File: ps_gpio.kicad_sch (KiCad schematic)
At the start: 12 parts, among them U1 XC7Z010-1CLG400C

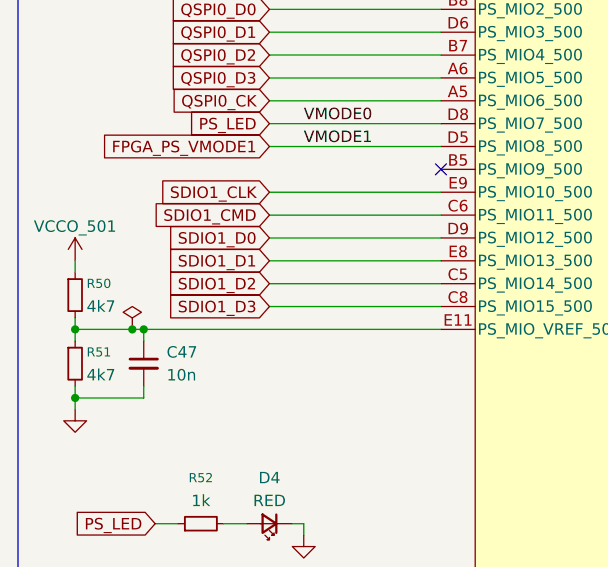
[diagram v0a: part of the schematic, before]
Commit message: update
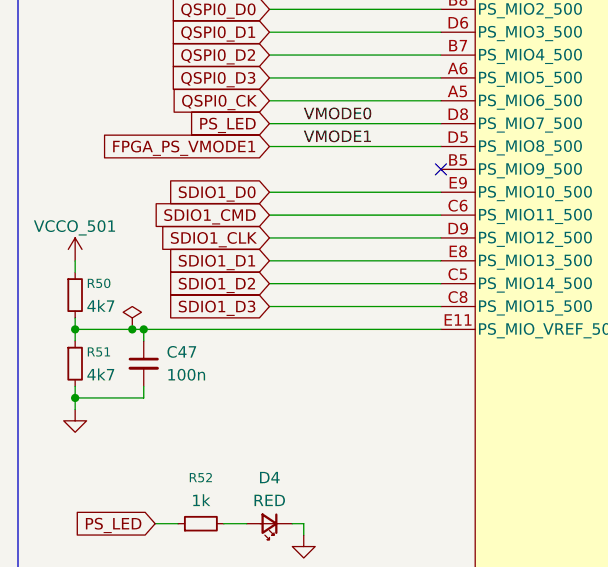
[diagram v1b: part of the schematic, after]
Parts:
- C47: value 10n -> 100n
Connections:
- net SDIO1_CLK: now also U1.D9 (PS_MIO12_500); no longer U1.E9 (PS_MIO10_500)
- net SDIO1_D0: now also U1.E9 (PS_MIO10_500); no longer U1.D9 (PS_MIO12_500)
